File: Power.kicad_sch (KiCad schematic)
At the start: 13 parts, among them J9 1935161, U1 LM2596DSADJG, U8 LM7805_TO220, U9 LM1117T-3.3

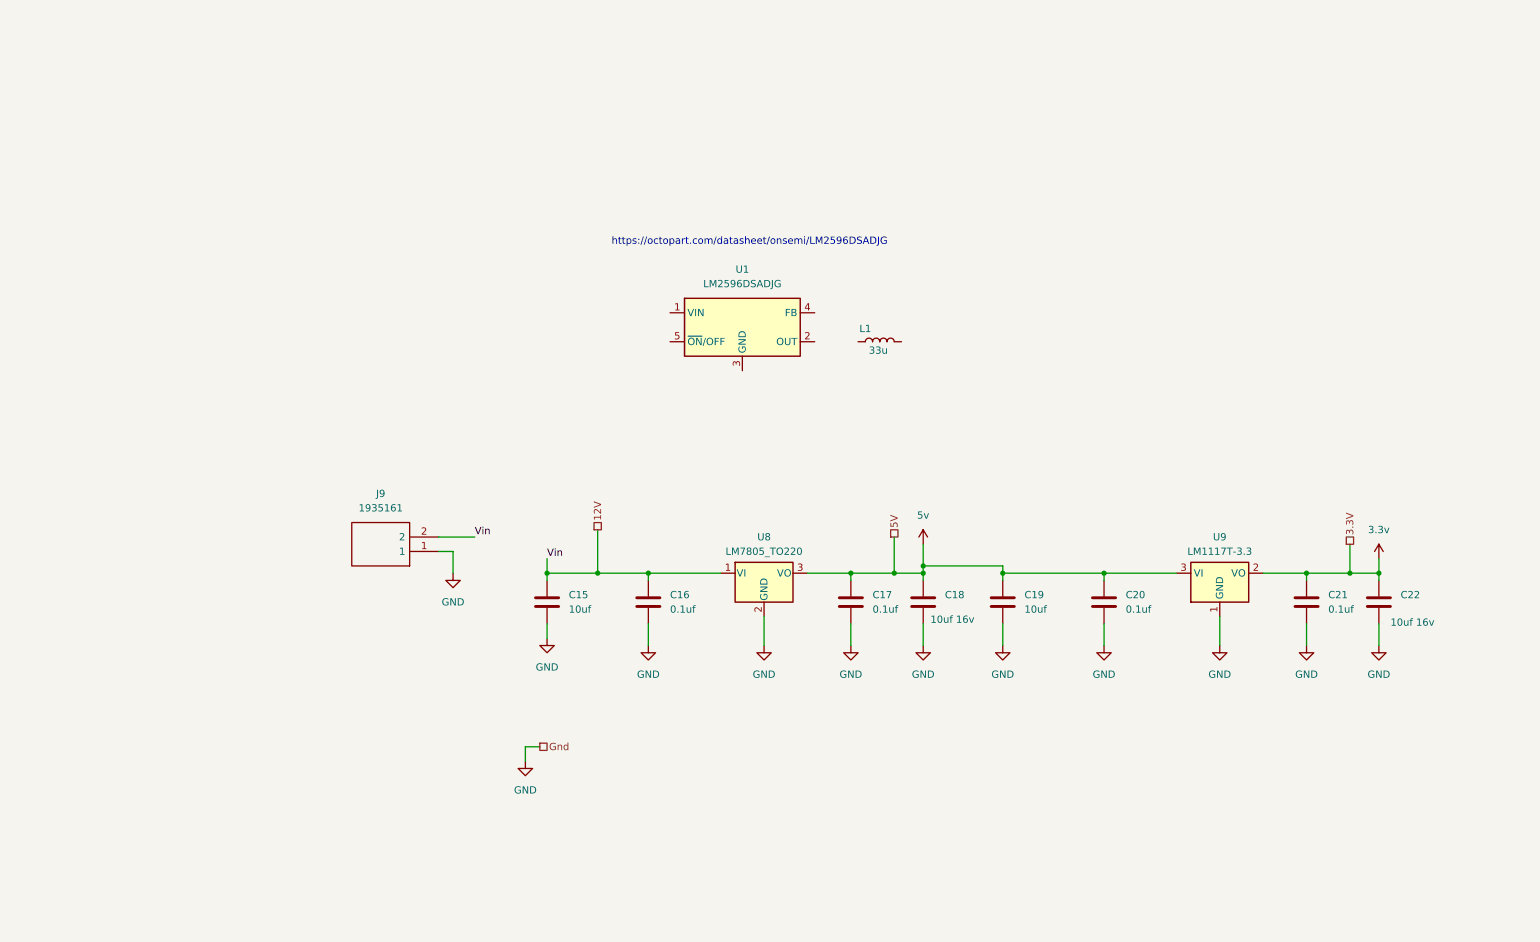
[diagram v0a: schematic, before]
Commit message: start adding switching pre-regulator
start isolating ground
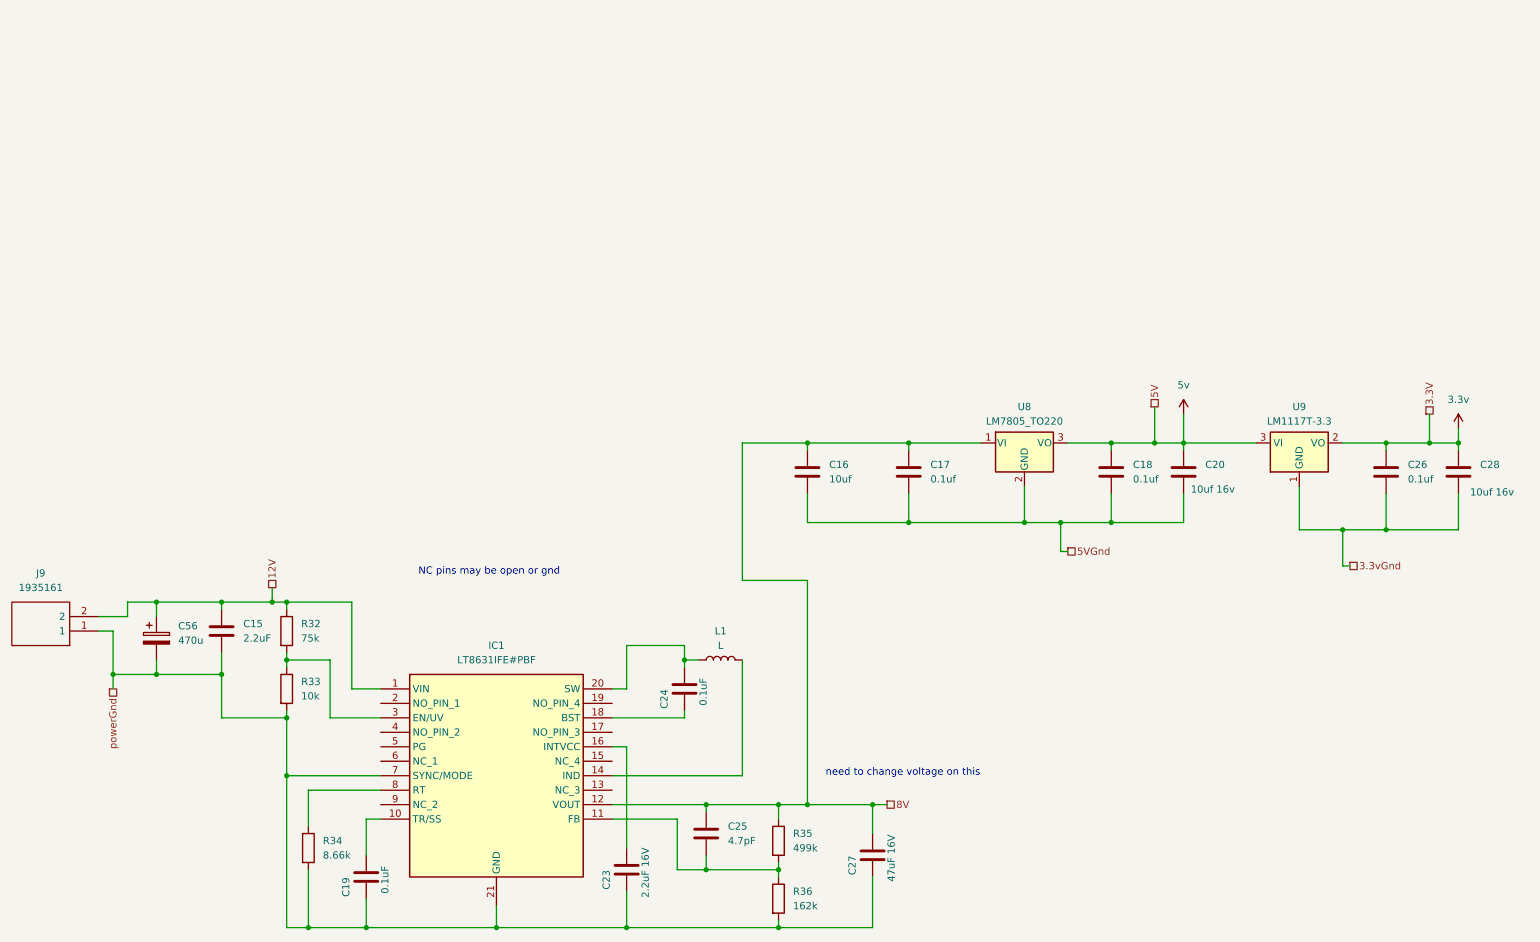
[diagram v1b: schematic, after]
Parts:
- removed C20: 0.1uf, Capacitor_SMD:C_0402_1005Metric, symbol Device:C
- removed U1: LM2596DSADJG, Package_TO_SOT_SMD:TO-263-5_TabPin3, symbol Regulator_Switching:LM2596S-ADJ
- added C15: 2.2uF, Capacitor_SMD:C_1206_3216Metric, symbol Device:C
- added C23: 2.2uF 16V, Capacitor_SMD:C_0805_2012Metric, symbol Device:C
- added C24: 0.1uF, Capacitor_SMD:C_0402_1005Metric, symbol Device:C
- added C25: 4.7pF, Capacitor_SMD:C_0402_1005Metric, symbol Device:C
- added C27: 47uF 16V, Capacitor_SMD:C_1210_3225Metric, symbol Device:C
- added C56: 470u, symbol Device:C_Polarized
- added IC1: LT8631IFE#PBF, SamacSys_Parts:SOP65P640X120-21N, symbol SamacSys_Parts:LT8631IFE#PBF
- added R32: 75k, Resistor_SMD:R_0402_1005Metric, symbol Device:R
- added R33: 10k, Resistor_SMD:R_0402_1005Metric, symbol Device:R
- added R34: 8.66k, Resistor_SMD:R_0402_1005Metric, symbol Device:R
- added R35: 499k, Resistor_SMD:R_0402_1005Metric, symbol Device:R
- added R36: 162k, Resistor_SMD:R_0402_1005Metric, symbol Device:R
- C19: value 10uf -> 0.1uF; Mouser (none) -> https://www.mouser.com/ProductDetail/TAIYO-YUDEN/MBASU105SB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
- L1: value 33u -> L
- renumbered C15 to C16, C16 to C17, C17 to C18, C18 to C20, C21 to C26, C22 to C28
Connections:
- net 12V: now also C15.1, C56.1, IC1.1 (VIN), R32.1; no longer C16.1, C17.1, U8.1 (VI)
- net 5v: no longer C19.1
- net at L1.1: now also C24.2, IC1.20 (SW)
- net at L1.2: now also IC1.14 (IND)
- net GND renamed 5VGnd
- net 5VGnd: no longer C19.2, C26.2, C28.2, J9.1, U9.1 (GND)
- new net: IC1.8 (RT), R34.1
- new net: C19.2, IC1.10 (TR/SS)
- new net: C25.2, IC1.11 (FB), R35.2, R36.1
- new net: C23.2, IC1.16 (INTVCC)
- new net: C24.1, IC1.18 (BST)
- new net: IC1.3 (EN/UV), R32.2, R33.1
- new net 3.3vGnd: C26.2, C28.2, U9.1 (GND)
- new net 8V: C16.1, C17.1, C25.1, C27.2, IC1.12 (VOUT), R35.1, U8.1 (VI)
- new net powerGnd: C15.2, C19.1, C23.1, C27.1, C56.2, IC1.21 (GND), IC1.7 (SYNC/MODE), J9.1, R33.2, R34.2, R36.2
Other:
- note added: "NC pins may be open or gnd"
- note added: "need to change voltage on this"
- note removed: "https://octopart.com/datasheet/onsemi/LM2596DSADJG"
- moved on the sheet: C16, C17, C18, C20, C26, C28, J9, U8, U9

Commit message: sch progress
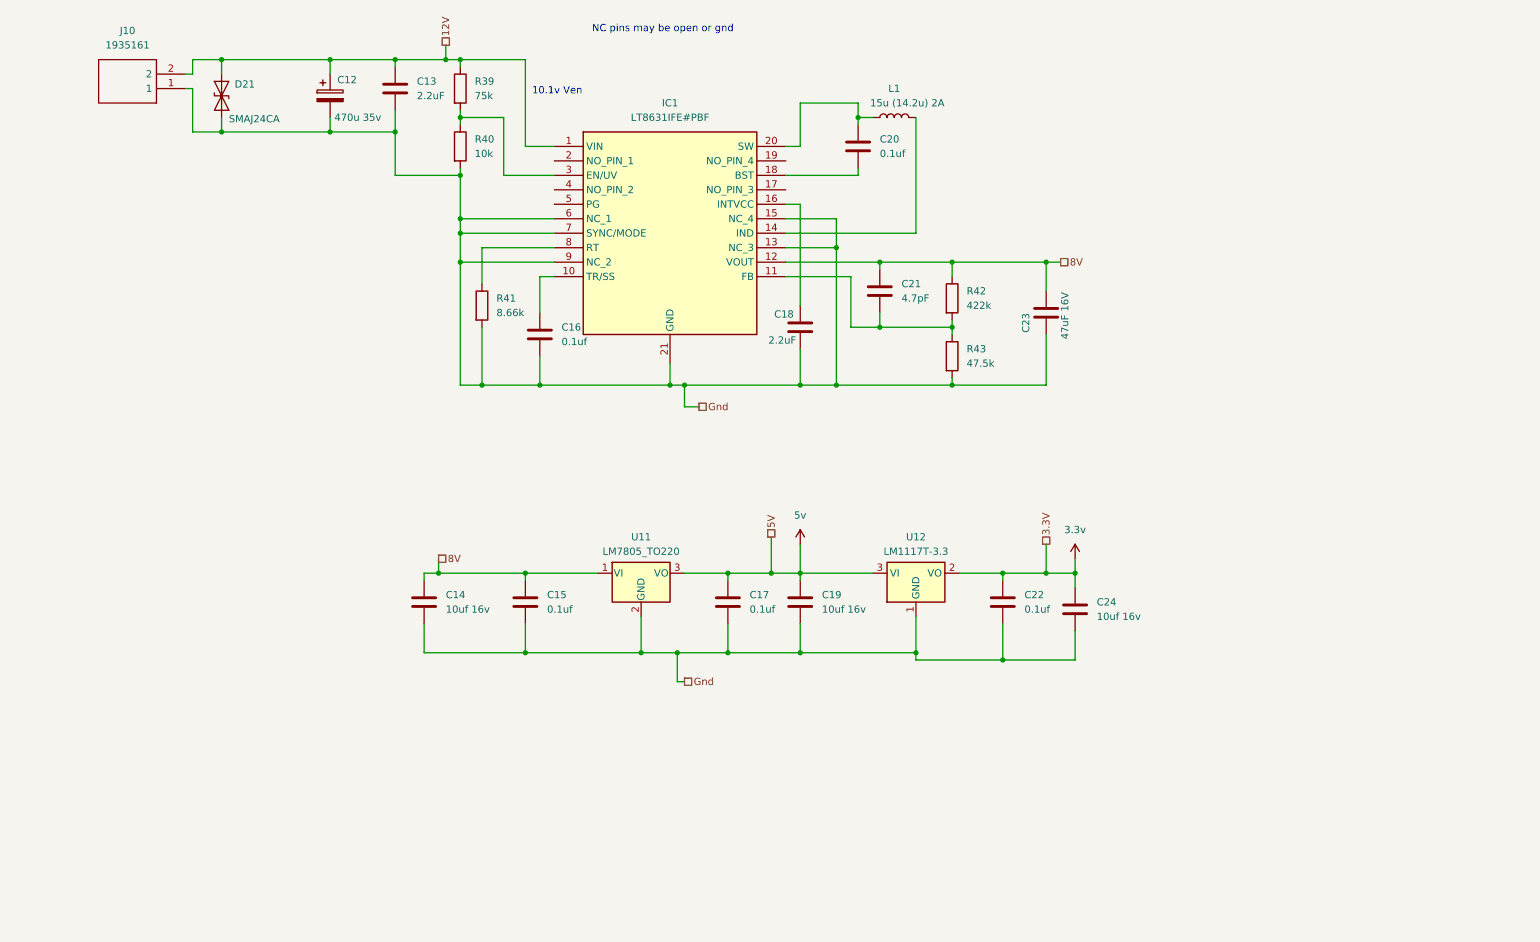
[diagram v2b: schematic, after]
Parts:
- removed C23: 2.2uF 16V, Capacitor_SMD:C_0805_2012Metric, symbol Device:C
- removed C26: 0.1uf, Capacitor_SMD:C_0402_1005Metric, symbol Device:C
- removed C28: 10uf 16v, Capacitor_SMD:C_0402_1005Metric, symbol Device:C
- added C14: 10uf 16v, Capacitor_SMD:C_0805_2012Metric, symbol Device:C
- added C15, C22: 0.1uf, Capacitor_SMD:C_0402_1005Metric, symbol Device:C
- added D21: SMAJ24CA, Diode_SMD:D_SMA, symbol Diode:SMAJ24CA
- C12: renamed from C56; value 470u -> 470u 35v; footprint (none) -> Capacitor_SMD:CP_Elec_10x14.3
- C16: value 10uf -> 0.1uf
- C18: value 0.1uf -> 2.2uF; footprint Capacitor_SMD:C_0402_1005Metric -> Capacitor_SMD:C_1206_3216Metric; Mouser (none) -> https://www.mouser.com/ProductDetail/Samsung-Electro-Mechan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
- C19, C24: value 0.1uF -> 10uf 16v; footprint Capacitor_SMD:C_0402_1005Metric -> Capacitor_SMD:C_0805_2012Metric; Mouser https://www.mouser.com/ProductDetail/TAIYO-YUDEN/MBASU105SB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 -> (none)
- C20: value 10uf 16v -> 0.1uf
- L1: value L -> 15u (14.2u) 2A; footprint (none) -> Inductor_SMD:L_Chilisin_BMRF00101040; part number (none) -> AMRM00101040150MA1
- R42: renamed from R35; value 499k -> 422k
- R43: renamed from R36; value 162k -> 47.5k
- renumbered C15 to C13, C25 to C21, C27 to C23, J9 to J10, R32 to R39, R33 to R40, R34 to R41, U8 to U11, U9 to U12
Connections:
- net 3.3vGnd is gone; now on net Gnd: U12.1 (GND)
- net 12V: now also D21.2 (A2)
- net 3.3v: now also C24.1, C22.1
- net 5v: now also C17.1, C19.1; no longer C18.1, C20.1
- net 8V: now also C14.1, C15.1; no longer C16.1, C17.1
- net at IC1.10 (TR/SS): now also C16.1; no longer C19.2
- net Gnd: now reaches IC1.13 (NC_3)
- net Gnd: now also C12.2, C13.2, C16.2, C17.2, C18.2, C19.2, C23.1, C24.2, IC1.15 (NC_4), IC1.21 (GND), IC1.6 (NC_1), IC1.7 (SYNC/MODE), IC1.9 (NC_2), J10.1, R40.2, R41.2, R43.2, U11.2 (GND), C14.2, C15.2, C22.2, D21.1 (A1)
- net at IC1.16 (INTVCC): now also C18.1
- net at IC1.18 (BST): now also C20.2; no longer C24.1
- net at IC1.20 (SW), L1.1: now also C20.1; no longer C24.2
- removed net 5VGnd: C16.2, C17.2, C18.2, C20.2, U11.2 (GND)
- removed net powerGnd: C12.2, C13.2, C19.1, C23.1, IC1.21 (GND), IC1.7 (SYNC/MODE), J10.1, R40.2, R41.2, R43.2
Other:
- note added: "10.1v Ven"
- note removed: "need to change voltage on this"
- moved on the sheet: C12, C13, C21, C23, IC1, J10, L1, R39, R40, R41, R42, R43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
